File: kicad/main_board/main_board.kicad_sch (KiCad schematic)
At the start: 8 parts

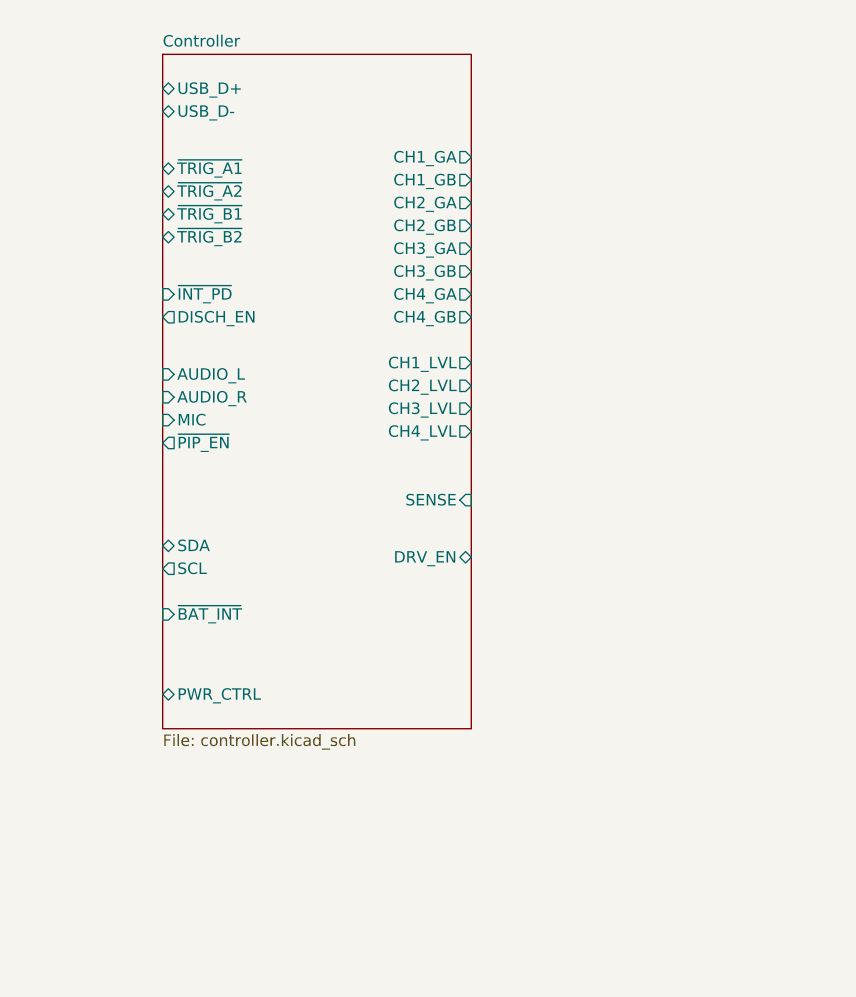
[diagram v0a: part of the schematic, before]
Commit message: add output
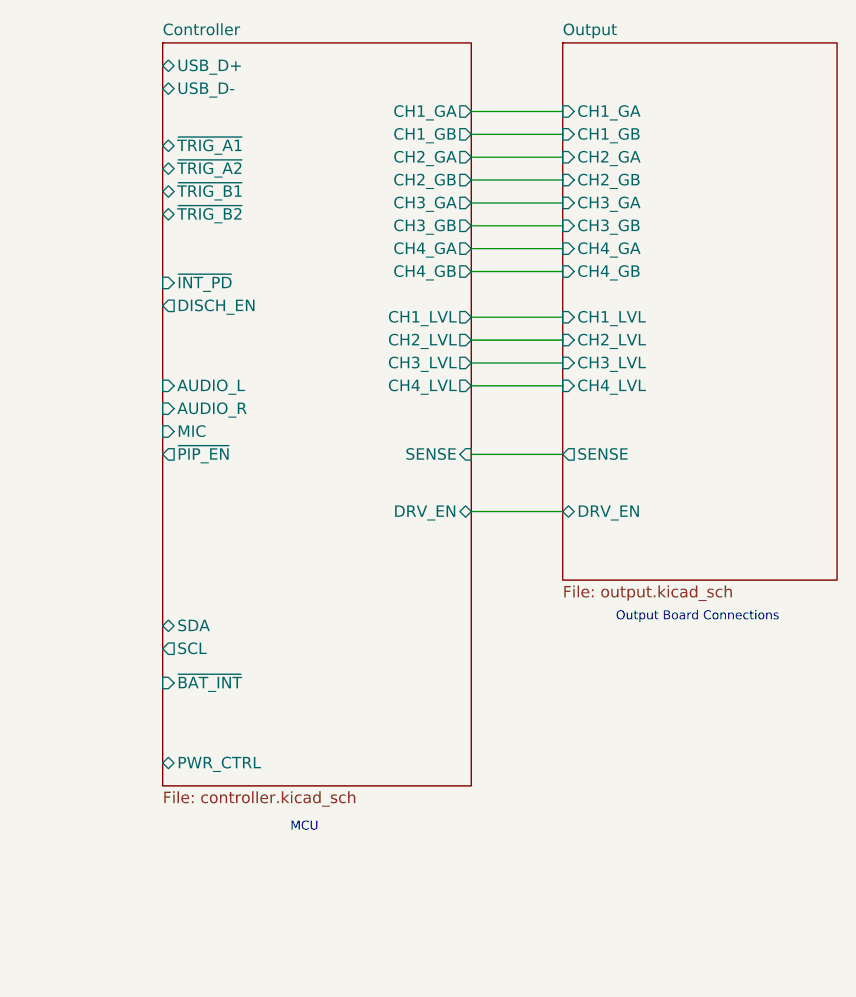
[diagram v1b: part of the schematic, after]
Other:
- added sheet Output (output.kicad_sch)
- note added: "MCU"
- note added: "Output Board Connections"
